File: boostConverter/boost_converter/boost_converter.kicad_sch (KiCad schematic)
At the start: 22 parts, among them IC1 TPS61175QPWPRQ1, J1 USB_C_Receptacle_PowerOnly_24P

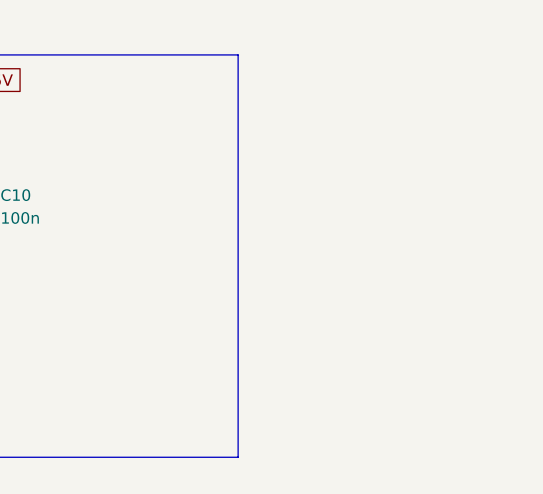
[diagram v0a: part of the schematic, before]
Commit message: update
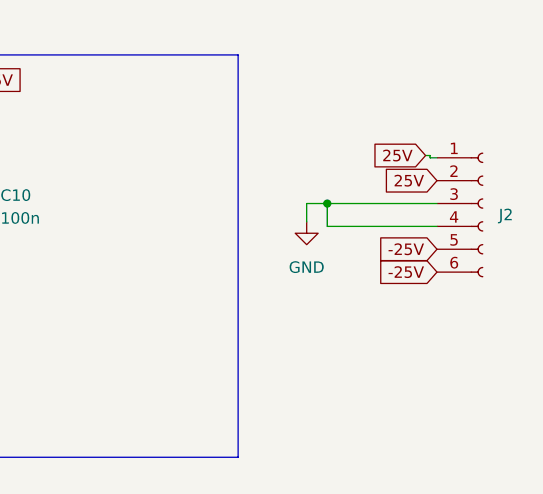
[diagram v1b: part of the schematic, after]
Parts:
- added J2: Conn_01x06_Socket, Connector_PinHeader_2.00mm:PinHeader_1x06_P2.00mm_Vertical, symbol Connector:Conn_01x06_Socket
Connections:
- net -25V: now also J2.5 (Pin_5), J2.6 (Pin_6)
- net 25V: now also J2.1 (Pin_1), J2.2 (Pin_2)
- net GND: now also J2.3 (Pin_3), J2.4 (Pin_4)
